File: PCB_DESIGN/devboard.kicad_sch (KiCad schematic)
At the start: 32 parts, among them J1 USB_C_Receptacle_USB2.0_14P, J2 Conn_02x18_Odd_Even, J3 Conn_02x18_Odd_Even, SW1 SW_Push, U1 RP2040, U2 NCP1117-3.3_SOT223, U3 W25Q128JVS, Y1 12 MHz

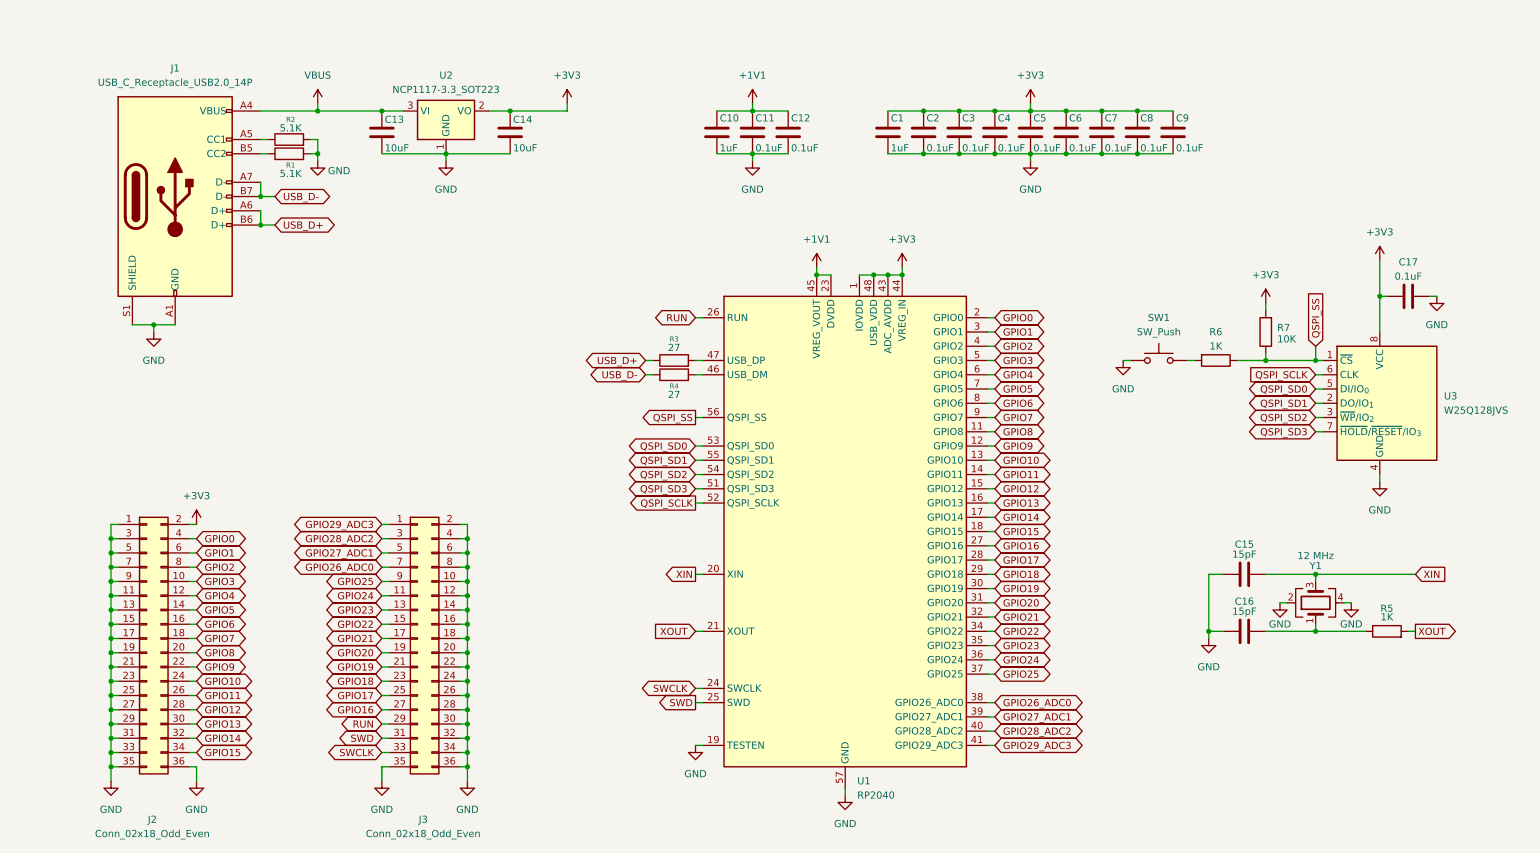
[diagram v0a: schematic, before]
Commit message: organizing schematic
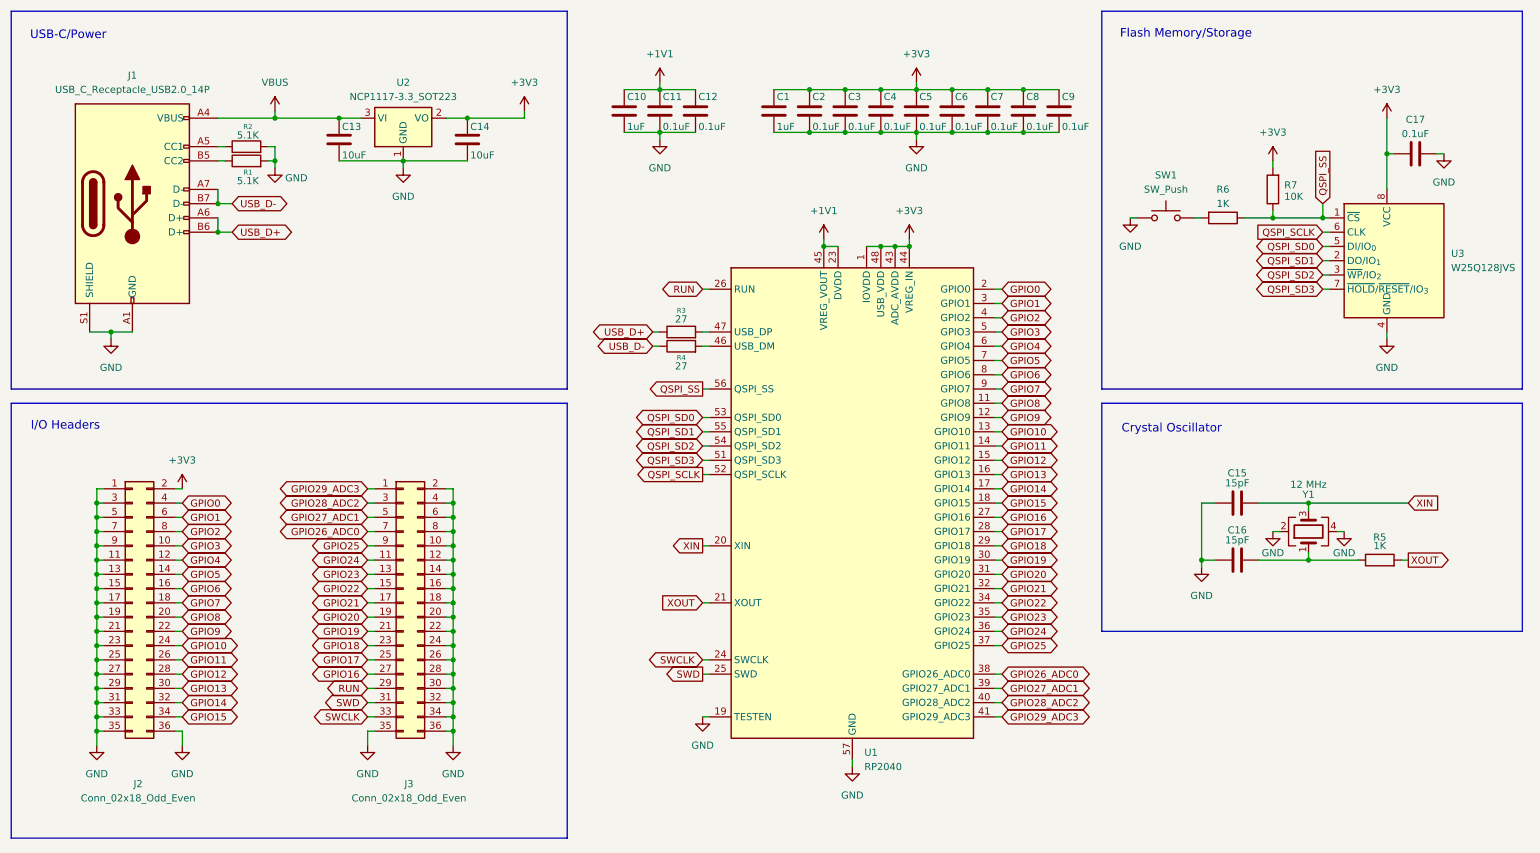
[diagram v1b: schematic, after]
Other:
- note added: "Crystal Oscillator"
- note added: "Flash Memory/Storage"
- note added: "I/O Headers"
- note added: "USB-C/Power"
- moved on the sheet: C1, C10, C11, C12, C13, C14, C15, C16, C17, C2, C3, C4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
